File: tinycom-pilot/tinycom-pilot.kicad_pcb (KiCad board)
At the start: 2 copper layers, 45.2 x 45.2 mm, 34 parts, among them J1 MICRO_SD_HINGE, P1 CONN_02X08, P2 CONN_02X08, P3 USB_A, P4 USB_OTG, U1 SY8008BAAC, U2 SY8008BAAC, U3 SY8008BAAC, U4 RTL8723BS(ComboModule)

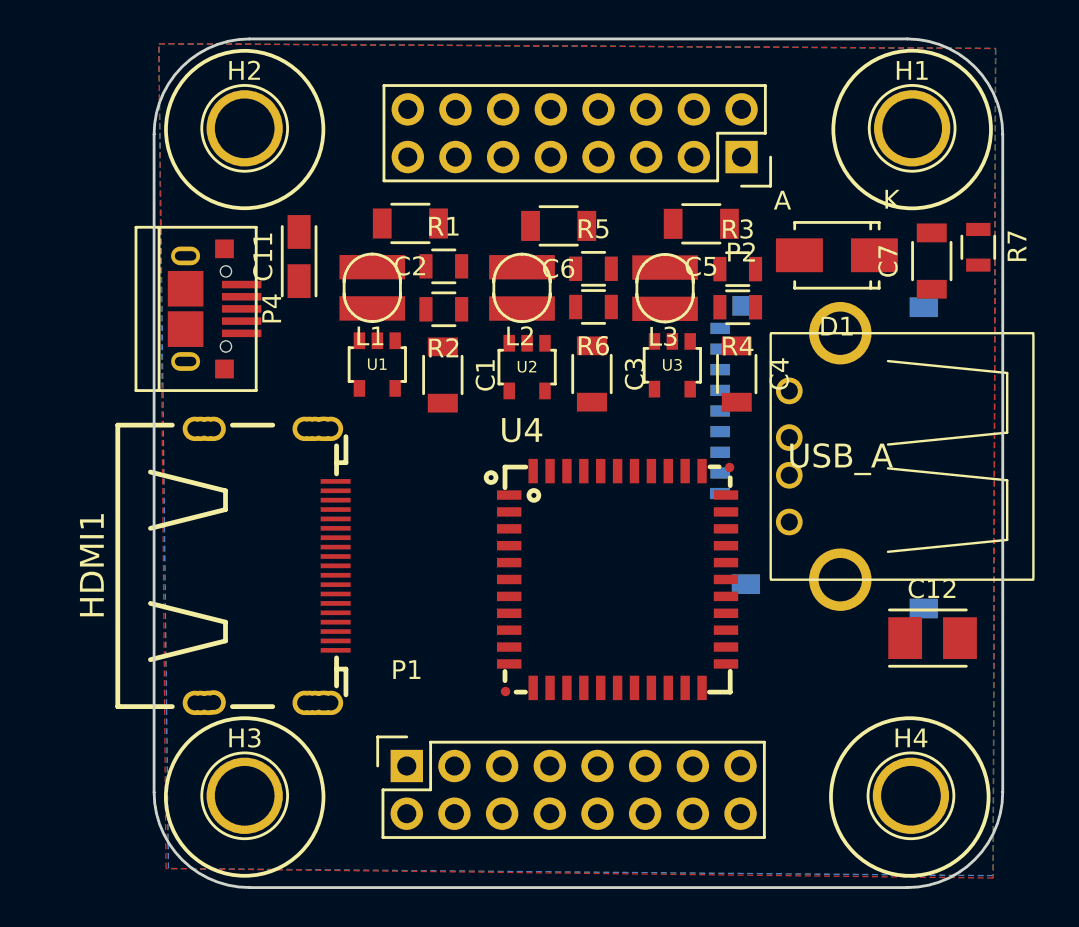
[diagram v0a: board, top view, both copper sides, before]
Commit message: pilot pic
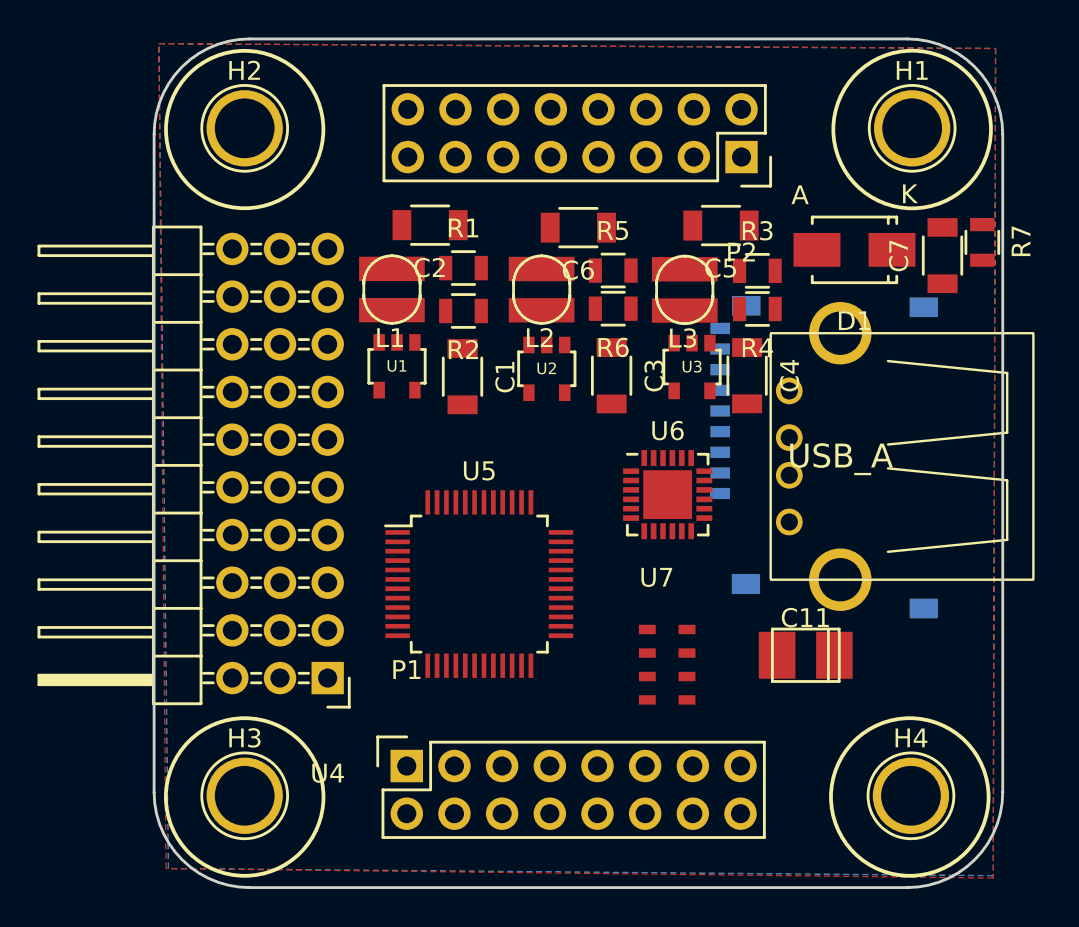
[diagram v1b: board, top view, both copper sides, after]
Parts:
- removed C12: CP_Small, Capacitors_Tantalum_SMD:TantalC_SizeB_EIA-3528_Reflow
- removed HDMI1: HDMI-SWM-19, tinycom:HDMI-SWM-19
- removed P4: USB_OTG, tinycom:tc-USB_Micro-B
- added U5: STM32-48PIN, Housings_QFP:LQFP-48_7x7mm_Pitch0.5mm, F.Cu at (141.8, 108.3)
- added U6: MPU6050, Housings_DFN_QFN:QFN-24-1EP_4x4mm_Pitch0.5mm, F.Cu at (151.8, 103.5)
- added U7: MS6511, tinycom:ms5611, F.Cu at (151.7, 112.7)
- C11: footprint Capacitors_Tantalum_SMD:TantalC_SizeA_EIA-3216_Reflow -> Capacitors_Tantalum_SMD:TantalC_SizeT_EIA-3528
- U4: value RTL8723BS(ComboModule) -> conn-3x10; footprint tinycom:RL-SM02BD(RTL8723BS) -> tinycom:Pin_Header_Angled_3x10
- moved C11 34.3 mm to (159.2, 112.1), turned to 0 degrees
- moved U4 16.3 mm to (133.7, 113.3), turned to 180 degrees
- moved C5 1.05 mm to (154.7, 89.2)
- moved C6 1.05 mm to (147.1, 89.3)
- moved L1 1.05 mm to (137.1, 92.6)
- moved R1 1.05 mm to (140.9, 91.5)
- moved R2 1.05 mm to (140.9, 93.7)
- moved R3 1.05 mm to (156.6, 91.6)
- moved R4 1.05 mm to (156.6, 93.6)
- moved U3 1.05 mm to (153.1, 96.7)
- moved L2 1.05 mm to (145.1, 92.6)
- moved C1 1.05 mm to (140.9, 97.2)
- moved C3 1.05 mm to (148.8, 97.2)
- moved R5 1.05 mm to (148.9, 91.6)
- moved R6 1.05 mm to (148.9, 93.6)
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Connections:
- P1 pad 14: UDP0 -> (no net)
- P1 pad 16: UDM0 -> (no net)
